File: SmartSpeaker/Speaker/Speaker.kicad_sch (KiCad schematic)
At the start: 26 parts, among them J1 Terminal_2, J2 Terminal_3, Q1 DMG2305UX-13, U1 LM384, U2 LM4040LP-3, U4 LTC1655LCN8

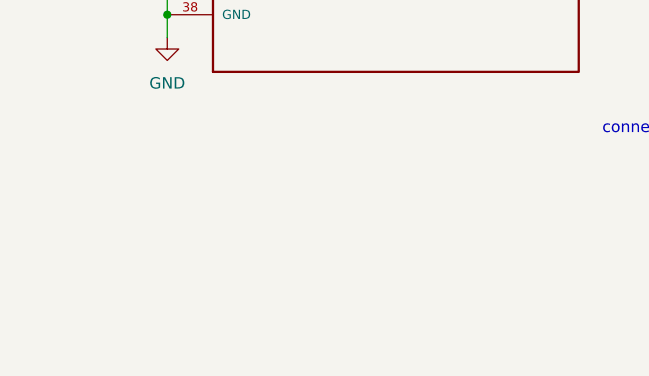
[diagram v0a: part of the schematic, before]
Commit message: lots of improvements, many semi-cosmetic
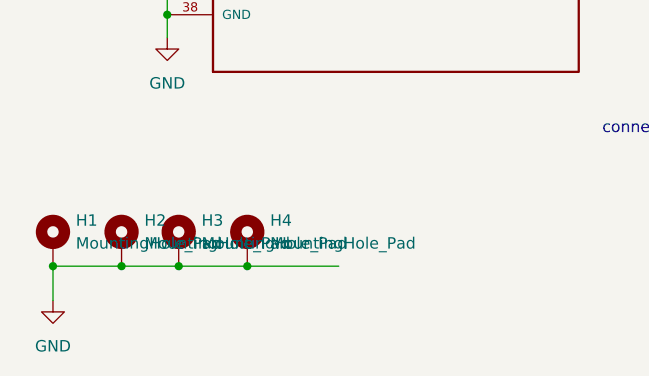
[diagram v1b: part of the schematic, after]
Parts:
- added H1, H2, H3, H4: MountingHole_Pad, MountingHole:MountingHole_3.2mm_M3_Pad, symbol Mechanical:MountingHole_Pad
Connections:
- net GND: now also H1.1, H2.1, H3.1, H4.1
